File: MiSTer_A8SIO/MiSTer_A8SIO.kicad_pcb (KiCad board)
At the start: 2 copper layers, 71 x 61.5 mm, 16 parts, among them J1 USB3_A, J2 SIO CONNECTOR, J3 Conn_01x10_Socket, J4 Conn_01x10_Socket, J5 Conn_01x02_Socket, J6 Conn_01x02_Socket, Q1 BC857, U1 TXS0108EPW, U2 AMS1117-3.3

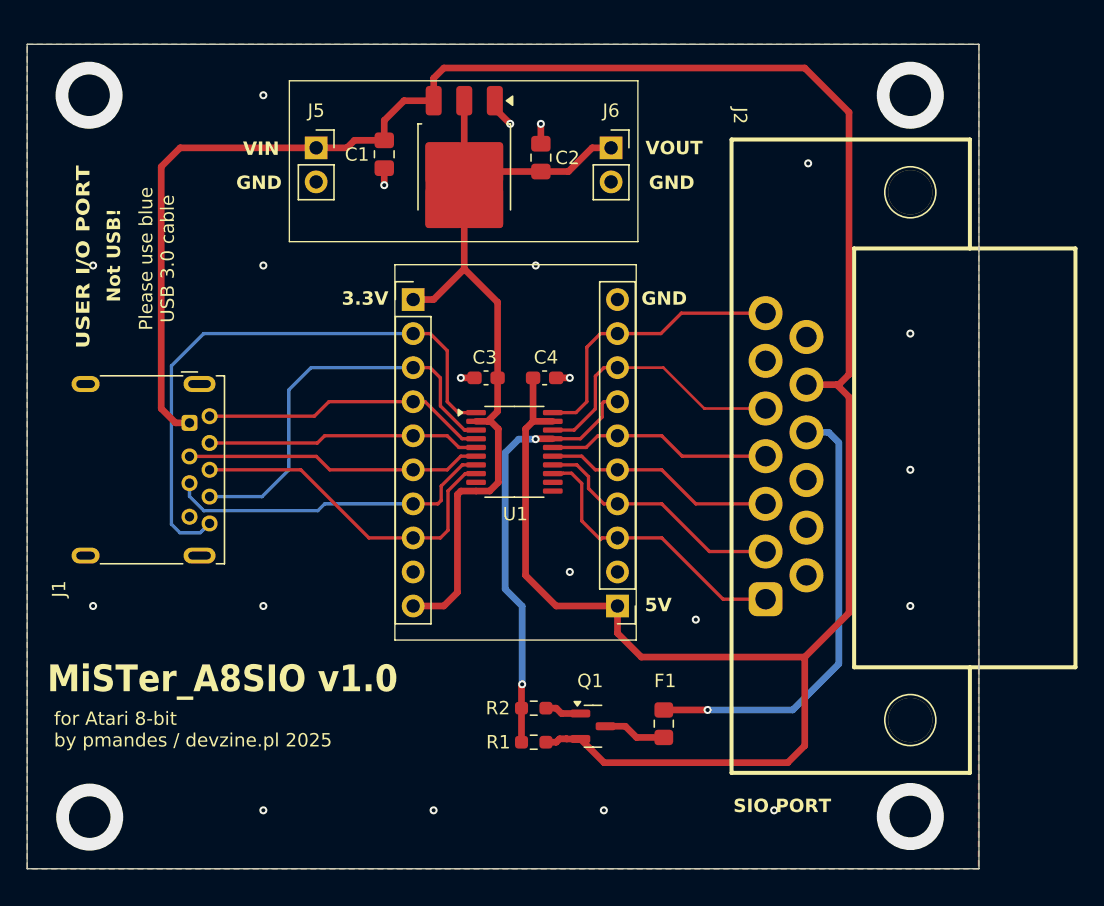
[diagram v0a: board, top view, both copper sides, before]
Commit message: Ver. 1.2, Fixed crossed lines
Signed-off-by: Pawel Mandes <pawel.mandes@gmail>
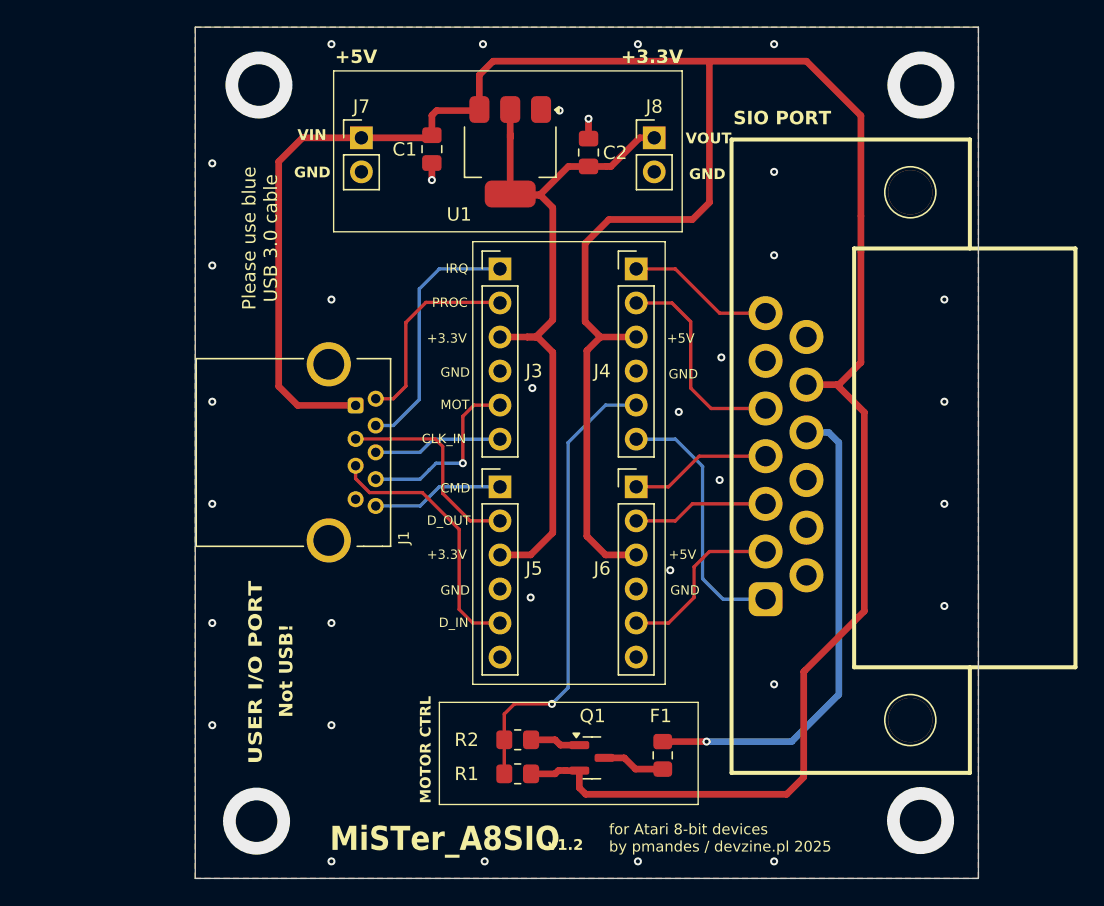
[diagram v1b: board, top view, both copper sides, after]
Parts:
- removed C3, C4: 100nF, Capacitor_SMD:C_0603_1608Metric_Pad1.08x0.95mm_HandSolder
- removed U2: AMS1117-3.3, Package_TO_SOT_SMD:TO-252-3_TabPin2
- added J7: Conn_01x02_Socket, Connector_PinHeader_2.54mm:PinHeader_1x02_P2.54mm_Vertical, F.Cu at (141.9, 54.0)
- added J8: Conn_01x02_Socket, Connector_PinHeader_2.54mm:PinHeader_1x02_P2.54mm_Vertical, F.Cu at (163.8, 54.0)
- added REF**: OSHW-Logo2_9.8x8mm_SilkScreen, Symbol:OSHW-Logo2_9.8x8mm_SilkScreen, B.Cu at (176.0, 102.9)
- C1, C2: value C -> 22uF
- J1: footprint Connector_USB:USB3_A_Molex_48393-001 -> Atari:USB3_A
- J3, J4: value Conn_01x10_Socket -> Conn_01x06_Socket; footprint Connector_PinHeader_2.54mm:PinHeader_1x10_P2.54mm_Vertical -> Connector_PinHeader_2.54mm:PinHeader_1x06_P2.54mm_Vertical
- J5, J6: value Conn_01x02_Socket -> Conn_01x06_Socket; footprint Connector_PinSocket_2.54mm:PinSocket_1x02_P2.54mm_Vertical -> Connector_PinHeader_2.54mm:PinHeader_1x06_P2.54mm_Vertical
- R1, R2: footprint Resistor_SMD:R_0603_1608Metric_Pad0.98x0.95mm_HandSolder -> Resistor_SMD:R_0805_2012Metric_Pad1.20x1.40mm_HandSolder
- U1: value TXS0108EPW -> AMS1117-3.3; footprint Package_SO:TSSOP-20_4.4x6.5mm_P0.65mm -> Package_TO_SOT_SMD:SOT-223
- moved J5 28.8 mm to (152.3, 80.0)
- moved J6 25.4 mm to (162.4, 80.0)
- moved J4 25.2 mm to (162.4, 63.8), turned to 0 degrees
- moved U1 22.4 mm to (153.0, 55.0), turned to -90 degrees
- moved J1 12.5 mm to (141.5, 73.9)
- moved J3 6.87 mm to (152.3, 63.8)
- moved C1 3.57 mm to (147.2, 54.8)
- moved C2 3.57 mm to (158.9, 55.1)
- moved R2 2.65 mm to (153.6, 98.9)
- moved R1 2.65 mm to (153.6, 101.4)
- moved F1 2.36 mm to (164.4, 100.0)
- moved Q1 2.36 mm to (159.1, 100.2)
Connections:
- J1 pad 5: /SIO_IRQ_A -> /SIO_CMD_A
- J1 pad 6: /SIO_PROC_A -> /SIO_MOTOR_A
- J1 pad 8: /SIO_CMD_A -> /SIO_IRQ_A
- J1 pad 9: /SIO_MOTOR_A -> /SIO_PROC_A
- J3 pad 1: +3.3V -> /SIO_IRQ_A
- J3 pad 2: /SIO_IRQ_A -> /SIO_PROC_A
- J3 pad 3: /SIO_PROC_A -> +3.3V
- J3 pad 4: /SIO_MOTOR_A -> GND
- J3 pad 5: /SIO_CMD_A -> /SIO_MOTOR_A
- J3 pad 6: /SIO_OUT_A -> /SIO_CLKIN_A
- J4 pad 1: VBUS -> /INTERRUPT
- J4 pad 2: unconnected-(J4-Pin_2-Pad2) -> /PROCEED
- J4 pad 3: /CLOCK IN -> VBUS
- J4 pad 4: /DATA IN -> GND
- J4 pad 5: /DATA OUT -> /PRE_MOTOR
- J4 pad 6: /COMMAND -> /CLOCK IN
- J5 pad 1: VBUS -> /SIO_CMD_A
- J5 pad 2: GND -> /SIO_OUT_A
- J6 pad 1: +3.3V -> /COMMAND
- J6 pad 2: GND -> /DATA OUT
- U1 pad 1: /SIO_IRQ_A -> GND
- U1 pad 3: /SIO_PROC_A -> VBUS
- U1 pad 4: /SIO_MOTOR_A -> +3.3V
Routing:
- net /SIO_IRQ_A: track 43.6 -> 18.9 mm
- net /SIO_CLKIN_A: track 25.7 -> 9.68 mm
- net /SIO_PROC_A: track 30.5 -> 15.0 mm
- net VBUS: track 191.8 -> 203.5 mm
- net /SIO_CMD_A: track 20.5 -> 9.86 mm
- net /INTERRUPT: track 21.3 -> 11.0 mm
- net +3.3V: track 63.8 -> 55.9 mm
- net /SIO_MOTOR_A: track 21.5 -> 13.6 mm, vias 0 -> 1
- net /DATA OUT: track 17.3 -> 10.2 mm
- net /SIO_OUT_A: track 22.2 -> 15.4 mm
- net /COMMAND: track 16.9 -> 10.6 mm
- net /DATA IN: track 19.1 -> 13.2 mm
- net /SIO_IN_A: track 24.8 -> 19.7 mm
- net /PROCEED: track 20.5 -> 15.8 mm
- net GND: track 6.73 -> 2.50 mm, vias 21 -> 33
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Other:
- board size 71 x 61.5 mm -> 58.4 x 63.5 mm
- board text added: "+3.3V"
- board text added: "+5V"
- board text added: "CLK_IN"
- board text added: "CMD"
- board text added: "D_IN"
- board text added: "D_OUT"
- board text added: "IRQ"
- board text added: "MOT"
- board text added: "MOTOR CTRL"
- board text added: "MiSTer_A8SIO"
- board text added: "MiSTer_A8SIO v1.2"
- board text added: "PROC"
- board text added: "SIO adapter for Atari 8-bit devices https://github.com/pmandes/MiSTer_A8SIO"
- board text added: "for Atari 8-bit devices by pmandes / devzine.pl 2025"
- board text added: "v1.2"
- board text removed: "3.3V"
- board text removed: "5V"
- board text removed: "MiSTer_A8SIO v1.0"
- board text removed: "for Atari 8-bit by pmandes / devzine.pl 2025"
